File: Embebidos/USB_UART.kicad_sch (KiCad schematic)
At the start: 9 parts, among them J1 USB_A, Q1 BC847, Q2 BC847

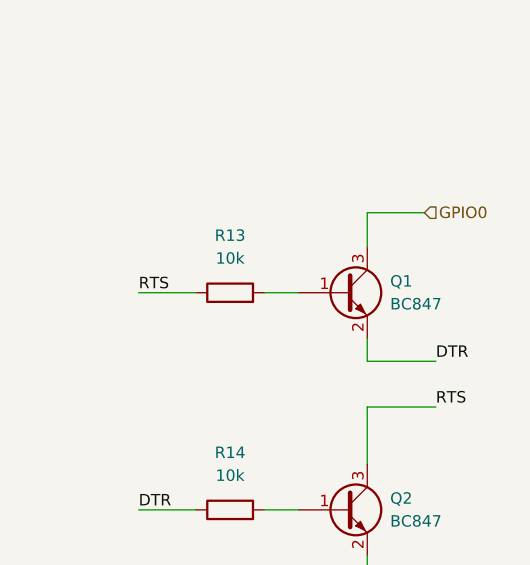
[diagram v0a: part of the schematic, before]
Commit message: aa
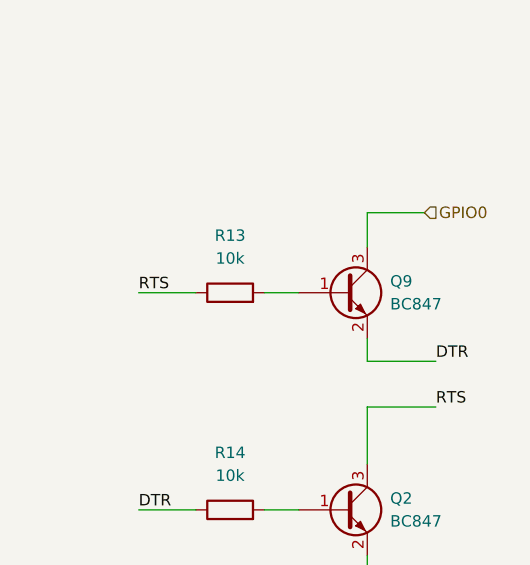
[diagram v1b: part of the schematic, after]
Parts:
- renumbered Q1 to Q9
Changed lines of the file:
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@@
   (symbol (lib_id "Transistor_BJT:BC847") (at 196.85 90.17 0) (unit 1)
     (in_bom yes) (on_board yes) (fields_autoplaced)
-    (property "Reference" "Q1" (id 0) (at 201.93 88.8999 0)
+    (property "Reference" "Q9" (id 0) (at 201.93 88.8999 0)
       (effects (font (size 1.27 1.27)) (justify left))
     )
